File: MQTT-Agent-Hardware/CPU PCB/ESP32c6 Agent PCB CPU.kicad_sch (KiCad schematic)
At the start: 19 parts, among them J1 Screw_Terminal_01x14, J10 Power, SW1 SW_Push, SW2 SW_Push, SW3 SW_Push, U2 DFPlayer_Module, U5 XIAO-ESP32-C6, U6 74AHCT125

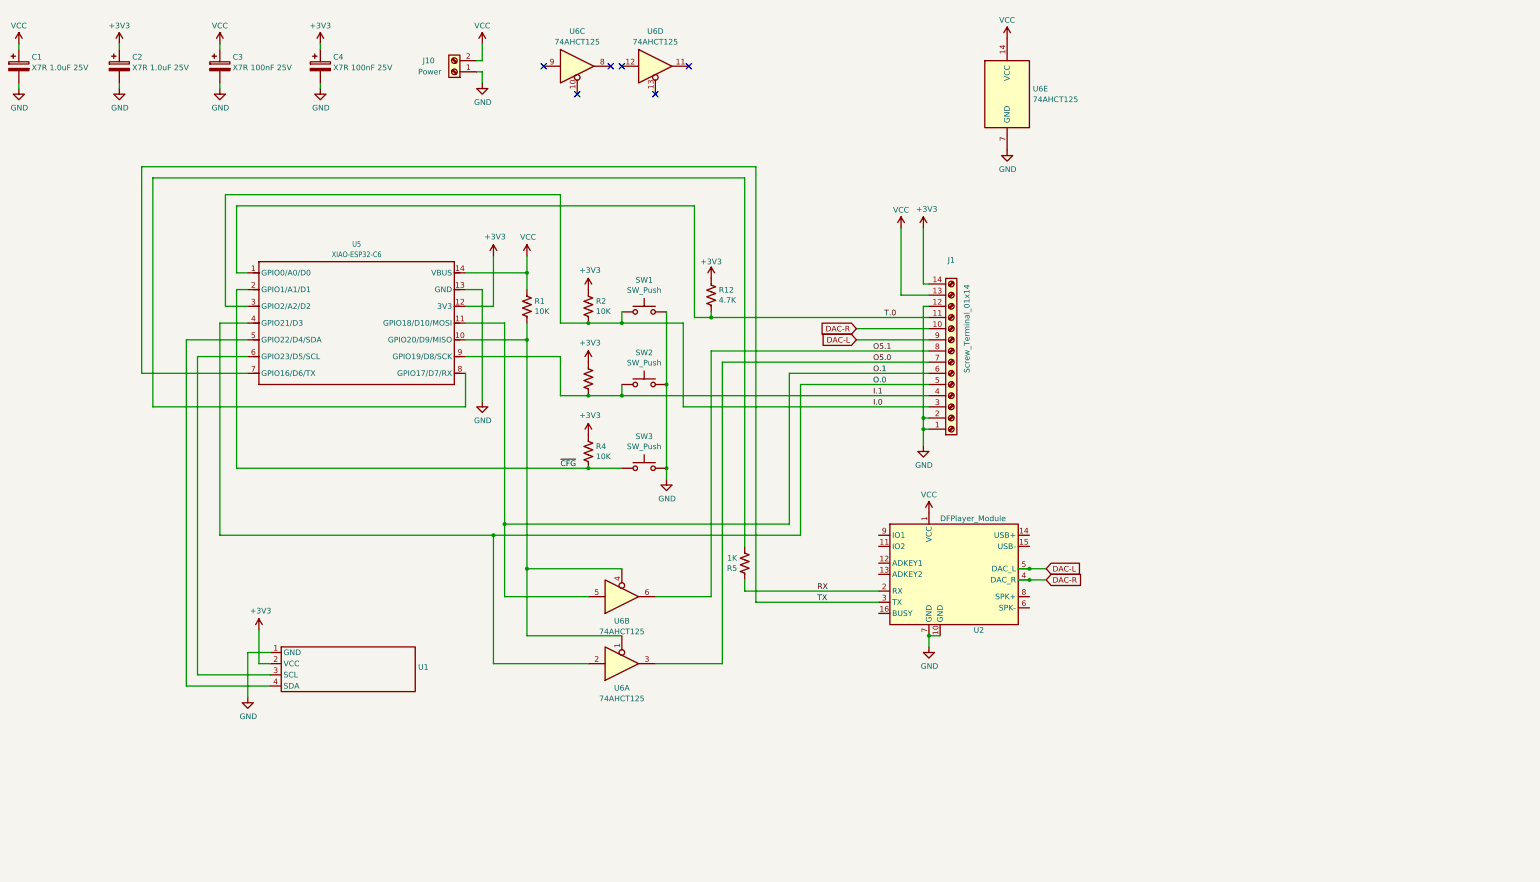
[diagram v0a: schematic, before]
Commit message: Cleanup and Finalize.
Updated footprints.
cleaned up silkscreen.
Changed schematic to B-size
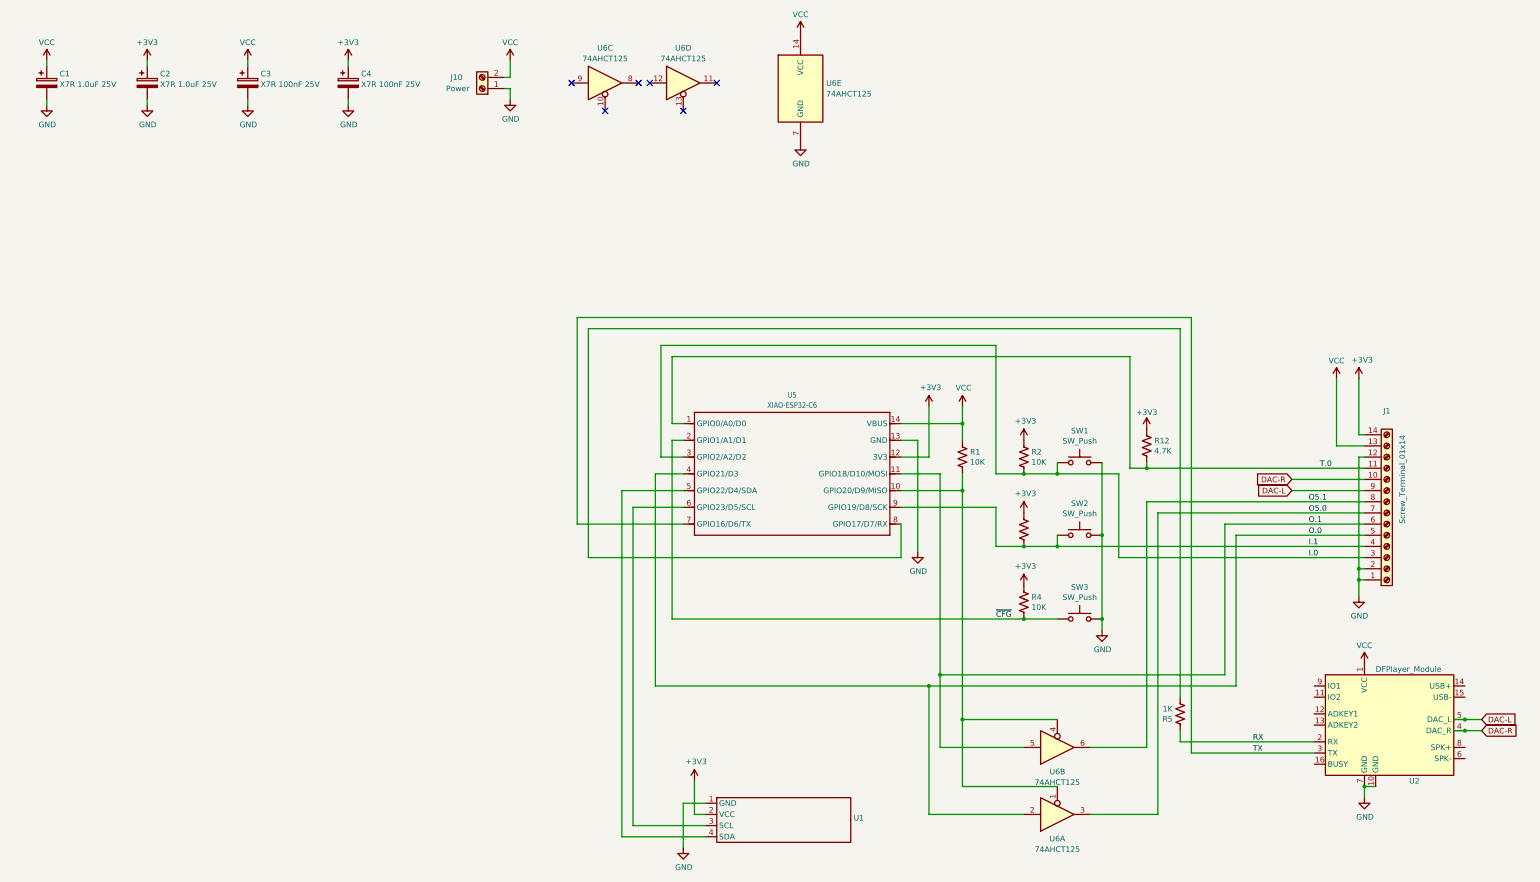
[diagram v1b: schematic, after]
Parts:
- U1: footprint MDS_Library:SSD1306-128x32 -> MDS_Library:SSD1306-128x32_Borderless
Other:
- moved on the sheet: C1, C2, C3, C4, J1, J10, R1, R12, R2, R4, R5, SW1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

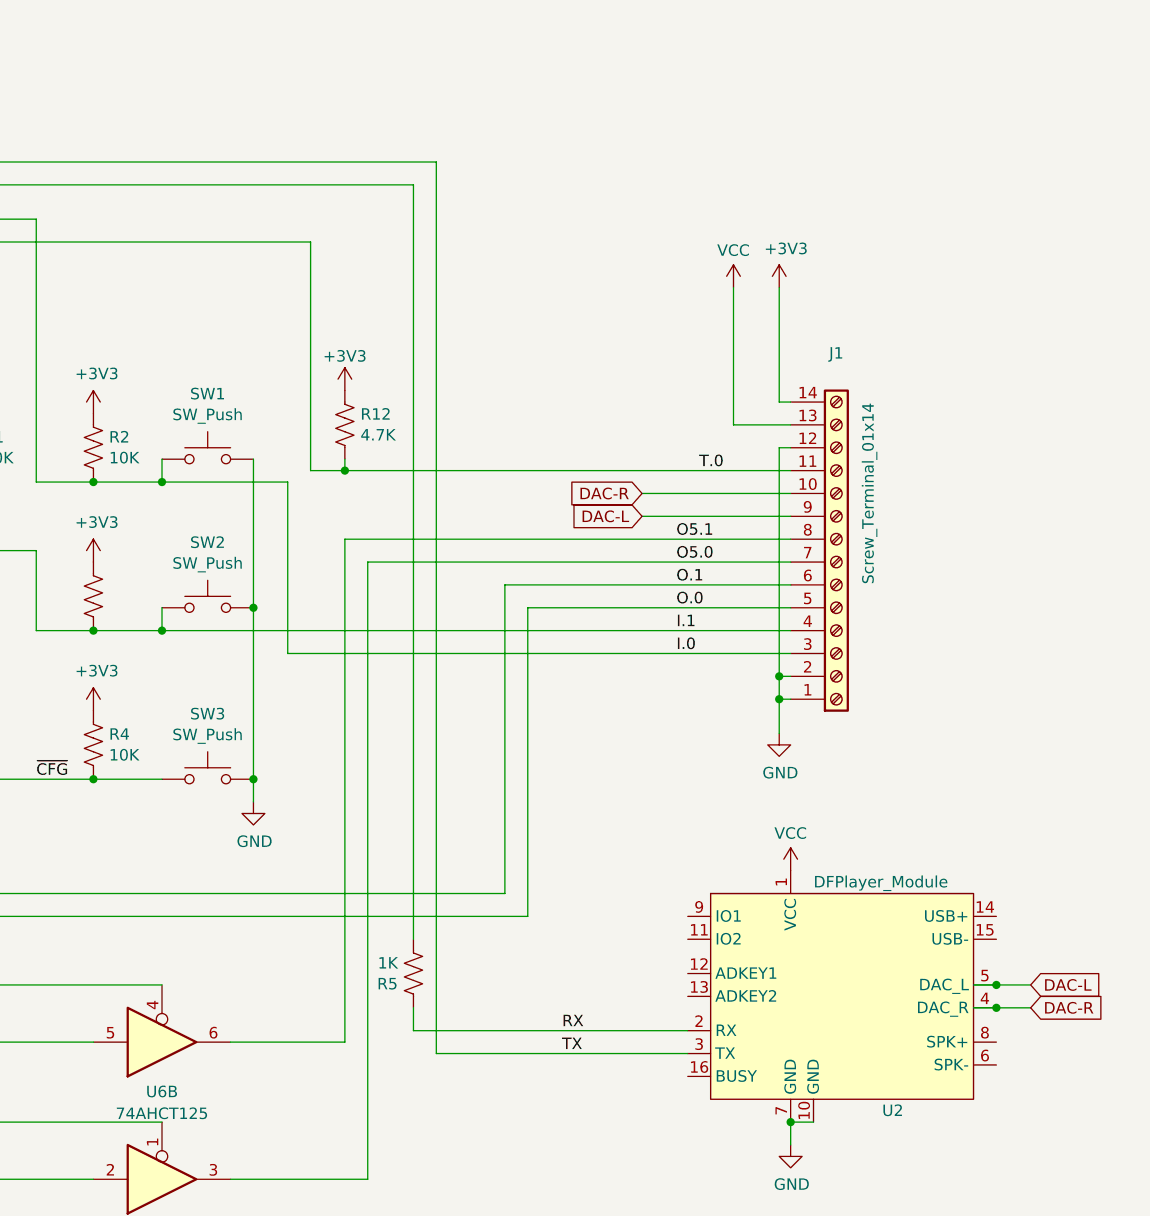
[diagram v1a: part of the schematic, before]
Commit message: Cleanup
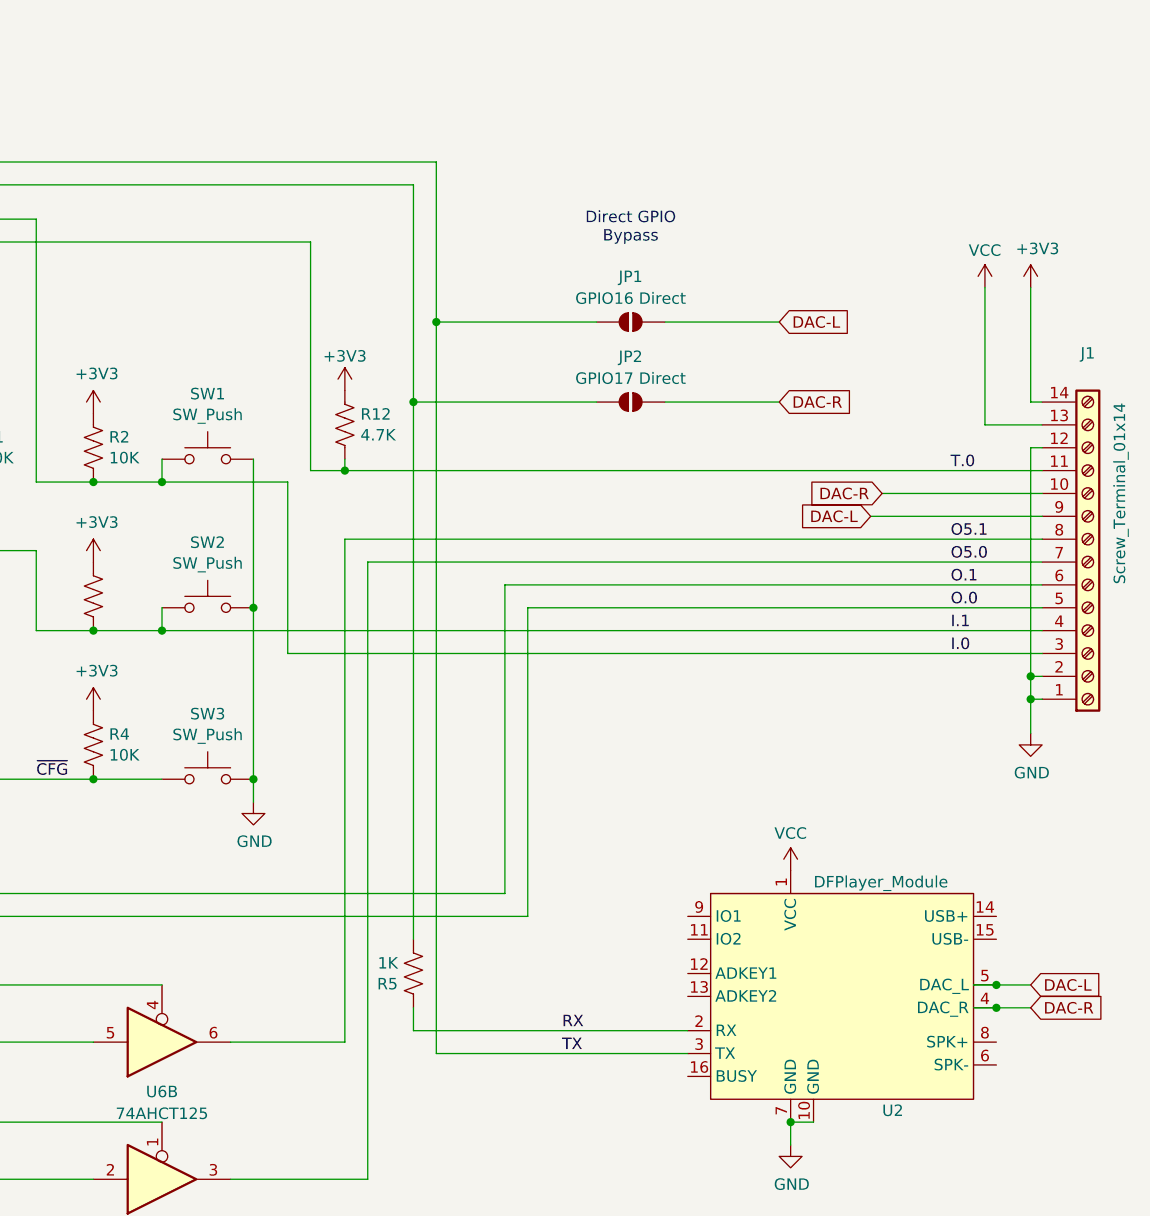
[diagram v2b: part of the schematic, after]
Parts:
- added JP1: GPIO16 Direct, Jumper:SolderJumper-2_P1.3mm_Open_Pad1.0x1.5mm, symbol Jumper:SolderJumper_2_Open
- added JP2: GPIO17 Direct, Jumper:SolderJumper-2_P1.3mm_Open_Pad1.0x1.5mm, symbol Jumper:SolderJumper_2_Open
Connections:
- net DAC-L: now also JP1.2 (B)
- net DAC-R: now also JP2.2 (B)
- net TX: now also JP1.1 (A)
- net at R5.2, U5.8 (GPIO17/D7/RX): now also JP2.1 (A)
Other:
- note added: "Direct GPIO Bypass"
- moved on the sheet: J1
